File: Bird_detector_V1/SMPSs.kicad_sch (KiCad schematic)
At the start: 25 parts, among them J12 enable, U16 TPS63020DSJR, U17 TPS63020DSJR

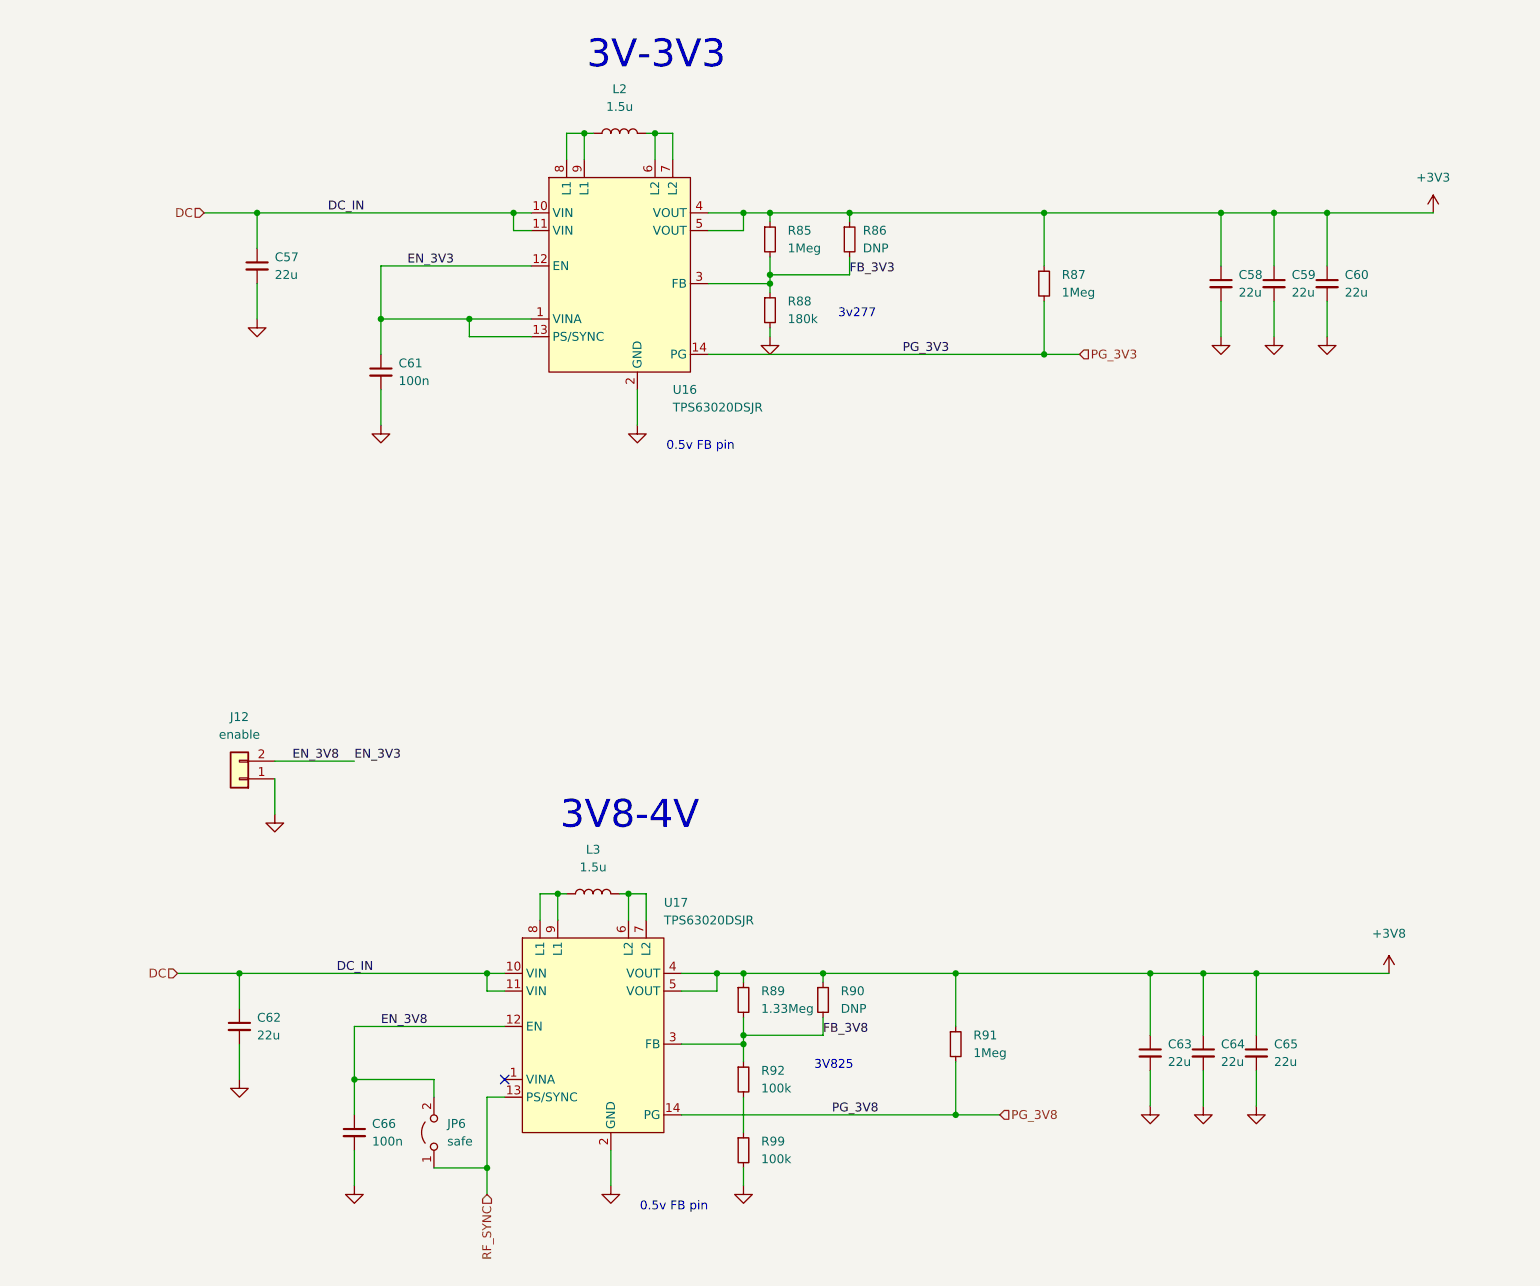
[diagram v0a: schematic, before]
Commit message: g
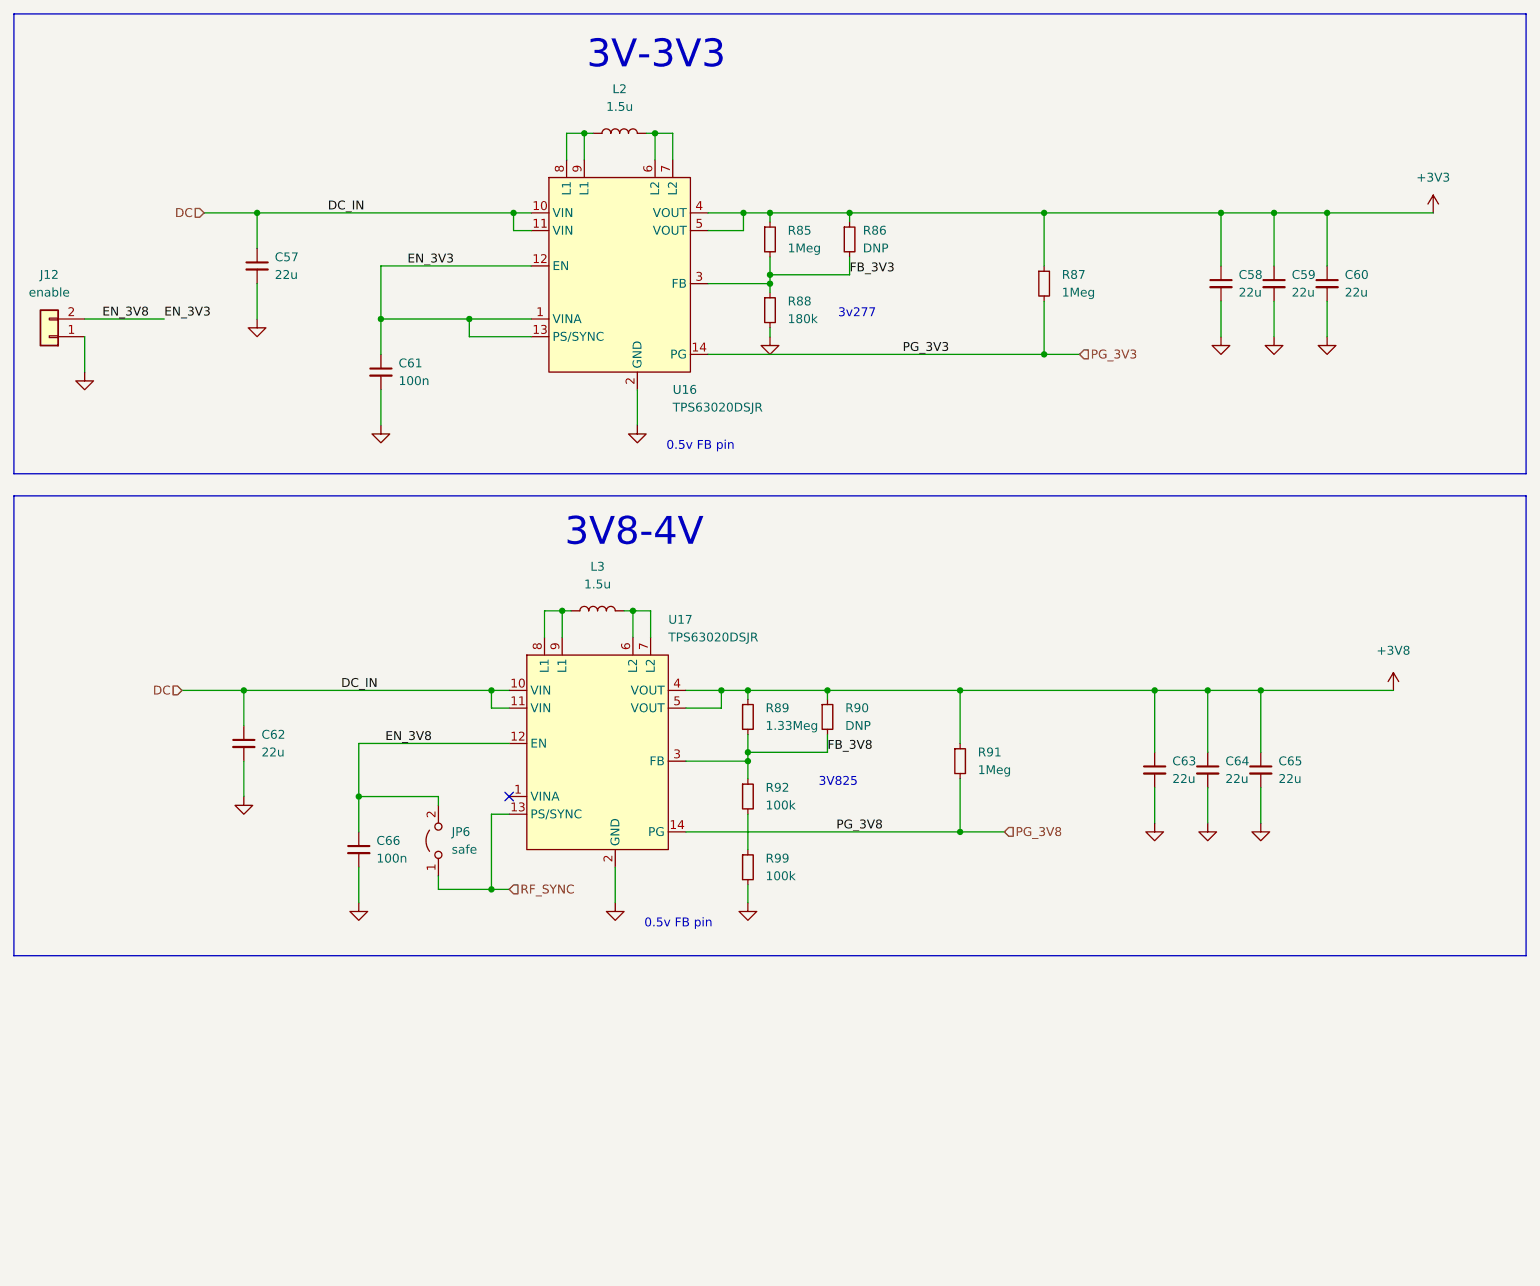
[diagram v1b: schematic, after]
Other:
- moved on the sheet: C62, C63, C64, C65, C66, J12, JP6, L3, R89, R90, R91, R92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
